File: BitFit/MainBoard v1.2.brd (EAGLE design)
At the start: 32.5 x 10.5 mm, 25 parts, among them J1 MICROUSB, U1 ATMEGA32U2QFN, U2 MCP738312, U3 LIS331, U5 REGULATOR

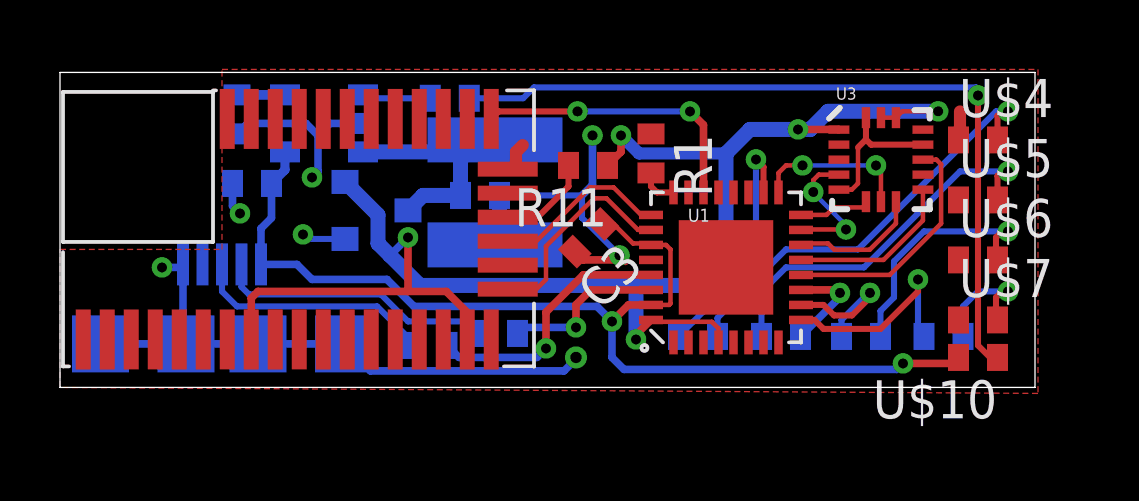
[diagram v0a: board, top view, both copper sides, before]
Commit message: File Clean Up v2
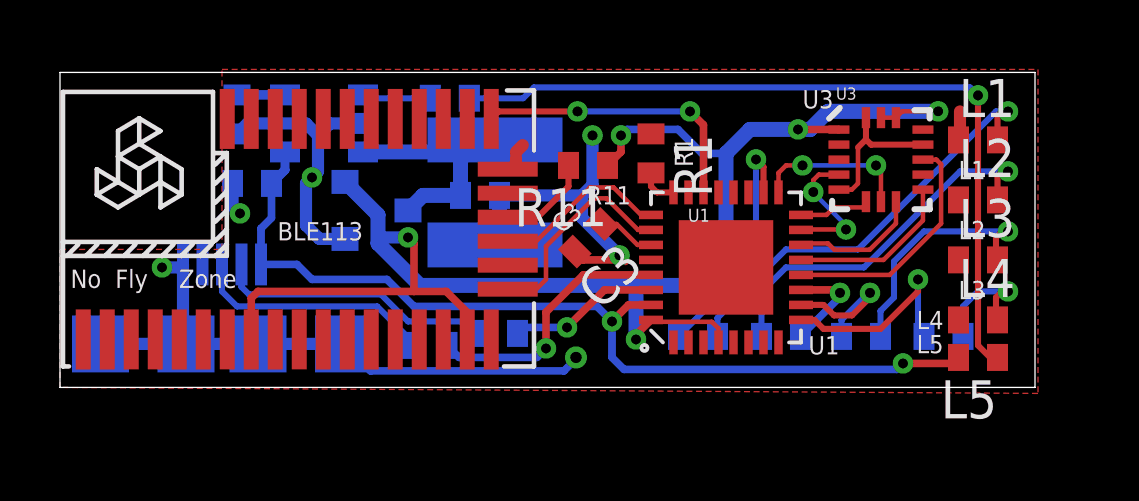
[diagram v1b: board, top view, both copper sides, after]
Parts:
- R4, R5, R6, R7, R9: value (none) -> 220ohm
- renumbered U$10 to L5, U$4 to L1, U$5 to L2, U$6 to L3, U$7 to L4
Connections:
- new net N$33: C3.1, U1.27
- net +5V: no longer C3.1, U1.27
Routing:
- net +5V: track 36.8 -> 31.7 mm
- net N$33: track 0.00 -> 1.91 mm
- net GND: track 47.3 -> 49.0 mm, vias 7 -> 6
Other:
- board text added: "BLE113"
- board text added: "C1"
- board text added: "C2"
- board text added: "C3"
- board text added: "L1"
- board text added: "L2"
- board text added: "L3"
- board text added: "L4"
- board text added: "L5"
- board text added: "LI-PO"
- board text added: "R1"
- board text added: "R11"
- board text added: "R2"
- board text added: "R3"
- board text added: "R4"
- board text added: "R5"
- board text added: "R6"
- board text added: "R7"
- board text added: "R8"
- board text added: "R9"
- board text added: "U1"
- board text added: "U2"
- board text added: "U3"
- board text added: "U5"
- board text added: "USB"
